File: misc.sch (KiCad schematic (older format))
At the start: 16 parts, among them J1 USB_OTG, U3 LP5900SDX-2.8, U4 AP7313-30SAG

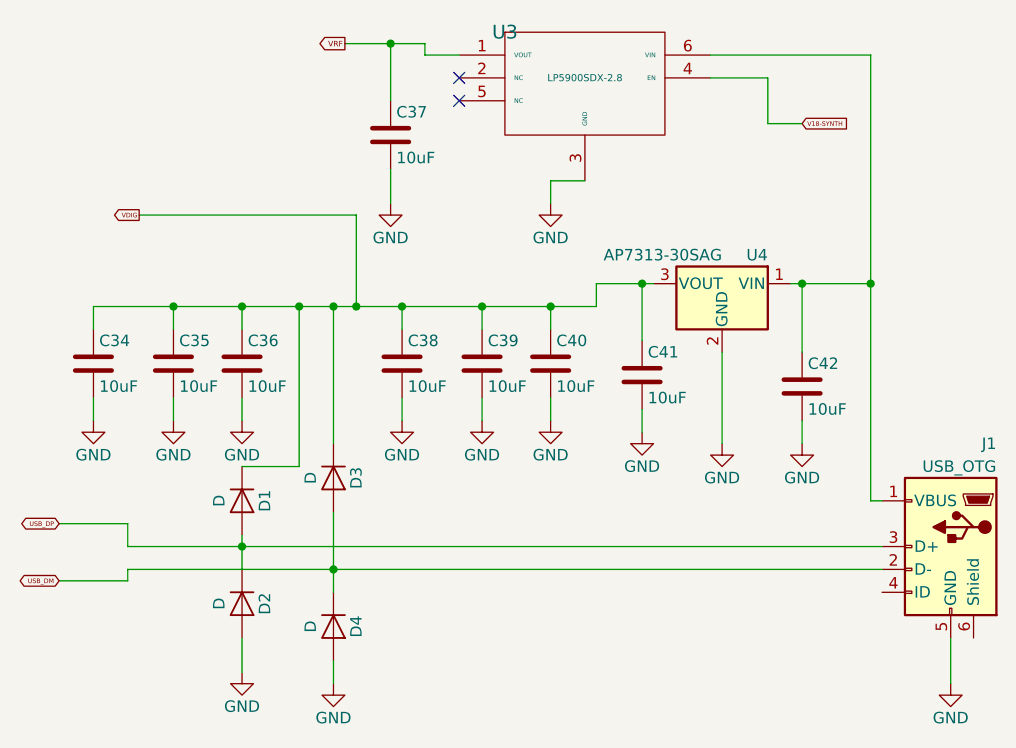
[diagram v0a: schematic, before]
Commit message: update and fix bug
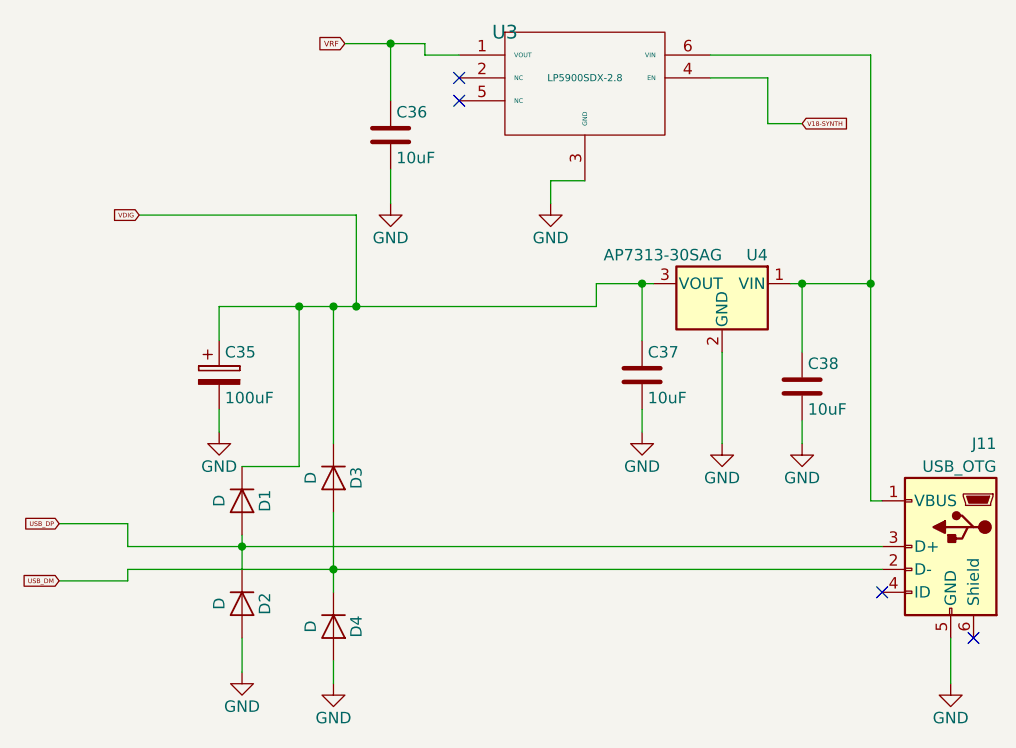
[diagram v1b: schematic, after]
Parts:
- removed C34, C35, C36, C38, C39, C40: 10uF, Capacitors_SMD:C_0805, symbol C
- added C35: 100uF, Capacitors_THT:CP_Radial_D5.0mm_P2.50mm, symbol CP
- C36: renamed from C37; footprint (none) -> Capacitors_SMD:C_0805
- D1: footprint (none) -> Diodes_SMD:D_0805
- renumbered C41 to C37, C42 to C38, J1 to J11
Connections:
- net GND: now also C35.2
- net VDIG: now also C35.1
- no-connect marks 2 -> 4
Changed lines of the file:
@@
 $EndDescr
-$Comp
-L C C34
-U 1 1 5C690AA3
-P 4050 2900
-F 0 "C34" H 4075 3000 50  0000 L CNN
-F 1 "10uF" H 4075 2800 50  0000 L CNN
-F 2 "Capacitors_SMD:C_0805" H 4088 2750 50  0001 C CNN
-F 3 "" H 4050 2900 50  0001 C CNN
-	1    4050 2900
-	1    0    0    -1
-$EndComp
-$Comp
-L C C35
-U 1 1 5C690ADC
-P 4400 2900
-F 0 "C35" H 4425 3000 50  0000 L CNN
-F 1 "10uF" H 4425 2800 50  0000 L CNN
-F 2 "Capacitors_SMD:C_0805" H 4438 2750 50  0001 C CNN
-F 3 "" H 4400 2900 50  0001 C CNN
-	1    4400 2900
-	1    0    0    -1
-$EndComp
-$Comp
-L C C36
-U 1 1 5C690B2D
-P 4700 2900
-F 0 "C36" H 4725 3000 50  0000 L CNN
-F 1 "10uF" H 4725 2800 50  0000 L CNN
-F 2 "Capacitors_SMD:C_0805" H 4738 2750 50  0001 C CNN
-F 3 "" H 4700 2900 50  0001 C CNN
-	1    4700 2900
-	1    0    0    -1
-$EndComp
-$Comp
-L C C38
-U 1 1 5C690C0C
-P 5400 2900
-F 0 "C38" H 5425 3000 50  0000 L CNN
-F 1 "10uF" H 5425 2800 50  0000 L CNN
-F 2 "Capacitors_SMD:C_0805" H 5438 2750 50  0001 C CNN
-F 3 "" H 5400 2900 50  0001 C CNN
-	1    5400 2900
-	1    0    0    -1
-$EndComp
-$Comp
-L C C39
-U 1 1 5C690C12
-P 5750 2900
-F 0 "C39" H 5775 3000 50  0000 L CNN
-F 1 "10uF" H 5775 2800 50  0000 L CNN
-F 2 "Capacitors_SMD:C_0805" H 5788 2750 50  0001 C CNN
-F 3 "" H 5750 2900 50  0001 C CNN
-	1    5750 2900
-	1    0    0    -1
-$EndComp
-$Comp
-L C C40
-U 1 1 5C690C18
-P 6050 2900
-F 0 "C40" H 6075 3000 50  0000 L CNN
-F 1 "10uF" H 6075 2800 50  0000 L CNN
-F 2 "Capacitors_SMD:C_0805" H 6088 2750 50  0001 C CNN
-F 3 "" H 6050 2900 50  0001 C CNN
-	1    6050 2900
-	1    0    0    -1
-$EndComp
 $Comp
 L D D1
@@
 F 0 "D1" H 4700 3600 50  0000 C CNN
 F 1 "D" H 4700 3400 50  0000 C CNN
-F 2 "" H 4700 3500 50  0001 C CNN
+F 2 "Diodes_SMD:D_0805" H 4700 3500 50  0001 C CNN
 F 3 "" H 4700 3500 50  0001 C CNN
 	1    4700 3500
@@
 $EndComp
 Wire Wire Line
-	4050 2750 4050 2650
-Wire Wire Line
-	4050 2650 6250 2650
-Wire Wire Line
-	6050 2650 6050 2750
-Wire Wire Line
-	5750 2750 5750 2650
-Connection ~ 5750 2650
-Wire Wire Line
-	5400 2750 5400 2650
-Connection ~ 5400 2650
-Wire Wire Line
-	4700 2750 4700 2650
-Connection ~ 4700 2650
-Wire Wire Line
-	4400 2750 4400 2650
-Connection ~ 4400 2650
+	4600 2650 6250 2650
 Wire Wire Line
 	5100 3250 5100 2650
@@
 Connection ~ 5100 3800
 $Comp
-L GND #PWR38
+L GND #PWR36
 U 1 1 5C690F71
 P 4700 4250
-F 0 "#PWR38" H 4700 4000 50  0001 C CNN
+F 0 "#PWR36" H 4700 4000 50  0001 C CNN
 F 1 "GND" H 4700 4100 50  0000 C CNN
 F 2 "" H 4700 4250 50  0001 C CNN
@@
 $EndComp
 $Comp
-L GND #PWR39
+L GND #PWR37
 U 1 1 5C690F9B
 P 5100 4300
-F 0 "#PWR39" H 5100 4050 50  0001 C CNN
+F 0 "#PWR37" H 5100 4050 50  0001 C CNN
 F 1 "GND" H 5100 4150 50  0000 C CNN
 F 2 "" H 5100 4300 50  0001 C CNN
@@
 Wire Wire Line
 	4950 3350 4950 2650
-Connection ~ 4950 2650
-Text GLabel 4250 2250 0    20   Output ~ 0
+Text GLabel 4250 2250 0    20   Input ~ 0
 VDIG
 Wire Wire Line
@@
 	5200 2250 5200 2650
 Connection ~ 5200 2650
-Text GLabel 3900 3850 0    20   BiDi ~ 0
+Text GLabel 3900 3850 0    20   Input ~ 0
 USB_DM
-Text GLabel 3900 3600 0    20   BiDi ~ 0
+Text GLabel 3900 3600 0    20   Input ~ 0
 USB_DP
 Wire Wire Line
@@
 L GND #PWR35
 U 1 1 5C6911FA
-P 4050 3150
-F 0 "#PWR35" H 4050 2900 50  0001 C CNN
-F 1 "GND" H 4050 3000 50  0000 C CNN
-F 2 "" H 4050 3150 50  0001 C CNN
-F 3 "" H 4050 3150 50  0001 C CNN
-	1    4050 3150
-	1    0    0    -1
-$EndComp
-$Comp
-L GND #PWR36
-U 1 1 5C691224
-P 4400 3150
-F 0 "#PWR36" H 4400 2900 50  0001 C CNN
-F 1 "GND" H 4400 3000 50  0000 C CNN
-F 2 "" H 4400 3150 50  0001 C CNN
-F 3 "" H 4400 3150 50  0001 C CNN
-	1    4400 3150
-	1    0    0    -1
-$EndComp
-$Comp
-L GND #PWR37
-U 1 1 5C69124E
-P 4700 3150
-F 0 "#PWR37" H 4700 2900 50  0001 C CNN
-F 1 "GND" H 4700 3000 50  0000 C CNN
-F 2 "" H 4700 3150 50  0001 C CNN
-F 3 "" H 4700 3150 50  0001 C CNN
-	1    4700 3150
-	1    0    0    -1
-$EndComp
-$Comp
-L GND #PWR41
-U 1 1 5C691278
-P 5400 3150
-F 0 "#PWR41" H 5400 2900 50  0001 C CNN
-F 1 "GND" H 5400 3000 50  0000 C CNN
-F 2 "" H 5400 3150 50  0001 C CNN
-F 3 "" H 5400 3150 50  0001 C CNN
-	1    5400 3150
-	1    0    0    -1
-$EndComp
-$Comp
-L GND #PWR42
-U 1 1 5C6912A2
-P 5750 3150
-F 0 "#PWR42" H 5750 2900 50  0001 C CNN
-F 1 "GND" H 5750 3000 50  0000 C CNN
-F 2 "" H 5750 3150 50  0001 C CNN
-F 3 "" H 5750 3150 50  0001 C CNN
-	1    5750 3150
-	1    0    0    -1
-$EndComp
-$Comp
-L GND #PWR44
-U 1 1 5C6912CC
-P 6050 3150
-F 0 "#PWR44" H 6050 2900 50  0001 C CNN
-F 1 "GND" H 6050 3000 50  0000 C CNN
-F 2 "" H 6050 3150 50  0001 C CNN
-F 3 "" H 6050 3150 50  0001 C CNN
-	1    6050 3150
-	1    0    0    -1
-$EndComp
-Wire Wire Line
-	6050 3150 6050 3050
-Wire Wire Line
-	5750 3150 5750 3050
-Wire Wire Line
-	5400 3150 5400 3050
-Wire Wire Line
-	4700 3150 4700 3050
-Wire Wire Line
-	4400 3150 4400 3050
-Wire Wire Line
-	4050 3150 4050 3050
+P 4600 3200
+F 0 "#PWR35" H 4600 2950 50  0001 C CNN
+F 1 "GND" H 4600 3050 50  0000 C CNN
+F 2 "" H 4600 3200 50  0001 C CNN
+F 3 "" H 4600 3200 50  0001 C CNN
+	1    4600 3200
+	1    0    0    -1
+$EndComp
 $Comp
 L AP2204R-3.0 U4
@@
 $EndComp
 $Comp
-L C C42
+L C C38
 U 1 1 5C691852
 P 7150 3000
-F 0 "C42" H 7175 3100 50  0000 L CNN
+F 0 "C38" H 7175 3100 50  0000 L CNN
 F 1 "10uF" H 7175 2900 50  0000 L CNN
 F 2 "Capacitors_SMD:C_0805" H 7188 2850 50  0001 C CNN
@@
 $EndComp
 $Comp
-L C C41
+L C C37
 U 1 1 5C6918BB
 P 6450 2950
-F 0 "C41" H 6475 3050 50  0000 L CNN
+F 0 "C37" H 6475 3050 50  0000 L CNN
 F 1 "10uF" H 6475 2850 50  0000 L CNN
 F 2 "Capacitors_SMD:C_0805" H 6488 2800 50  0001 C CNN
@@
 	7150 2550 7150 2850
 $Comp
-L GND #PWR46
+L GND #PWR41
 U 1 1 5C691B40
 P 6800 3250
-F 0 "#PWR46" H 6800 3000 50  0001 C CNN
+F 0 "#PWR41" H 6800 3000 50  0001 C CNN
 F 1 "GND" H 6800 3100 50  0000 C CNN
 F 2 "" H 6800 3250 50  0001 C CNN
@@
 Wire Wire Line
 	6250 2650 6250 2550
-Connection ~ 6050 2650
 Connection ~ 6450 2550
-Wire Wire Line
-	7450 3500 7500 3500
 Wire Wire Line
 	7450 1550 7450 3500
 Connection ~ 7150 2550
 $Comp
-L GND #PWR45
+L GND #PWR40
 U 1 1 5C692086
 P 6450 3200
-F 0 "#PWR45" H 6450 2950 50  0001 C CNN
+F 0 "#PWR40" H 6450 2950 50  0001 C CNN
 F 1 "GND" H 6450 3050 50  0000 C CNN
 F 2 "" H 6450 3200 50  0001 C CNN
@@
 $EndComp
 $Comp
-L GND #PWR47
+L GND #PWR42
 U 1 1 5C6920B8
 P 7150 3250
-F 0 "#PWR47" H 7150 3000 50  0001 C CNN
+F 0 "#PWR42" H 7150 3000 50  0001 C CNN
 F 1 "GND" H 7150 3100 50  0000 C CNN
 F 2 "" H 7150 3250 50  0001 C CNN
@@
 	7150 3250 7150 3150
 $Comp
-L GND #PWR43
+L GND #PWR39
 U 1 1 5C69221A
 P 6050 2200
-F 0 "#PWR43" H 6050 1950 50  0001 C CNN
+F 0 "#PWR39" H 6050 1950 50  0001 C CNN
 F 1 "GND" H 6050 2050 50  0000 C CNN
 F 2 "" H 6050 2200 50  0001 C CNN
@@
 	1    0    0    -1
 $EndComp
-Text GLabel 5150 1500 0    24   Output ~ 0
+Text GLabel 5150 1500 0    24   Input ~ 0
 VRF
 Wire Wire Line
@@
 NoConn ~ 5650 1750
 $Comp
-L C C37
+L C C36
 U 1 1 5C69264E
 P 5350 1900
-F 0 "C37" H 5375 2000 50  0000 L CNN
+F 0 "C36" H 5375 2000 50  0000 L CNN
 F 1 "10uF" H 5375 1800 50  0000 L CNN
-F 2 "" H 5388 1750 50  0001 C CNN
+F 2 "Capacitors_SMD:C_0805" H 5388 1750 50  0001 C CNN
 F 3 "" H 5350 1900 50  0001 C CNN
 	1    5350 1900
@@
 Connection ~ 5350 1500
 $Comp
-L GND #PWR40
+L GND #PWR38
 U 1 1 5C692712
 P 5350 2200
-F 0 "#PWR40" H 5350 1950 50  0001 C CNN
+F 0 "#PWR38" H 5350 1950 50  0001 C CNN
 F 1 "GND" H 5350 2050 50  0000 C CNN
 F 2 "" H 5350 2200 50  0001 C CNN
@@
 	6050 2100 6050 2200
 $Comp
-L GND #PWR48
+L GND #PWR43
 U 1 1 5C693D92
 P 7800 4300
-F 0 "#PWR48" H 7800 4050 50  0001 C CNN
+F 0 "#PWR43" H 7800 4050 50  0001 C CNN
 F 1 "GND" H 7800 4150 50  0000 C CNN
 F 2 "" H 7800 4300 50  0001 C CNN
@@
 	7800 4300 7800 4100
 $Comp
-L USB_OTG J1
+L USB_OTG J11
 U 1 1 5C695F80
 P 7800 3700
-F 0 "J1" H 7600 4150 50  0000 L CNN
+F 0 "J11" H 7600 4150 50  0000 L CNN
 F 1 "USB_OTG" H 7600 4050 50  0000 L CNN
 F 2 "Connectors:USB_Mini-B" H 7950 3650 50  0001 C CNN
@@
 	1    0    0    -1
 $EndComp
+NoConn ~ 7500 3900
+NoConn ~ 7900 4100
+Wire Wire Line
+	7450 3500 7500 3500
+Wire Wire Line
+	4600 2650 4600 2800
+Connection ~ 4950 2650
+$Comp
+L CP C35
+U 1 1 5C6ADA0A
+P 4600 2950
+F 0 "C35" H 4625 3050 50  0000 L CNN
+F 1 "100uF" H 4625 2850 50  0000 L CNN
+F 2 "Capacitors_THT:CP_Radial_D5.0mm_P2.50mm" H 4638 2800 50  0001 C CNN
+F 3 "" H 4600 2950 50  0001 C CNN
+	1    4600 2950
+	1    0    0    -1
+$EndComp
+Wire Wire Line
+	4600 3200 4600 3100
 $EndSCHEMATC
